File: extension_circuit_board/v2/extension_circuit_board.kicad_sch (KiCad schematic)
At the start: 9 parts, among them J1 GPIO_odd, J2 Jetson_Nano_GPIO, J3 GPIO_even, J4 FeatherWing_DCmotor, J5 PiOLED 2x3, J6 Motor Power, J7 Battery, SW1 SW_SPDT, U1 DFR0753

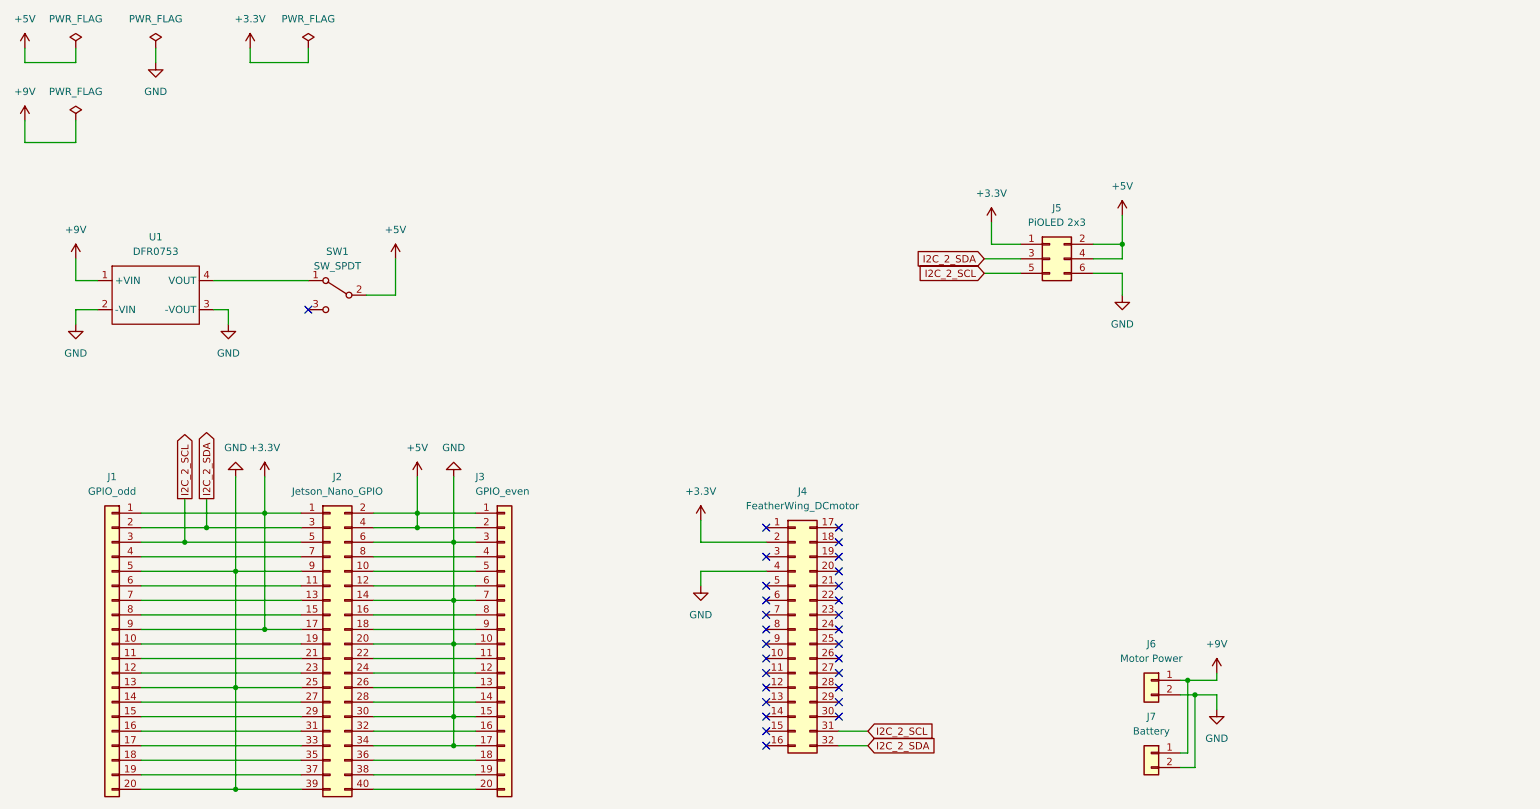
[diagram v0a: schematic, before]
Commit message: Updated
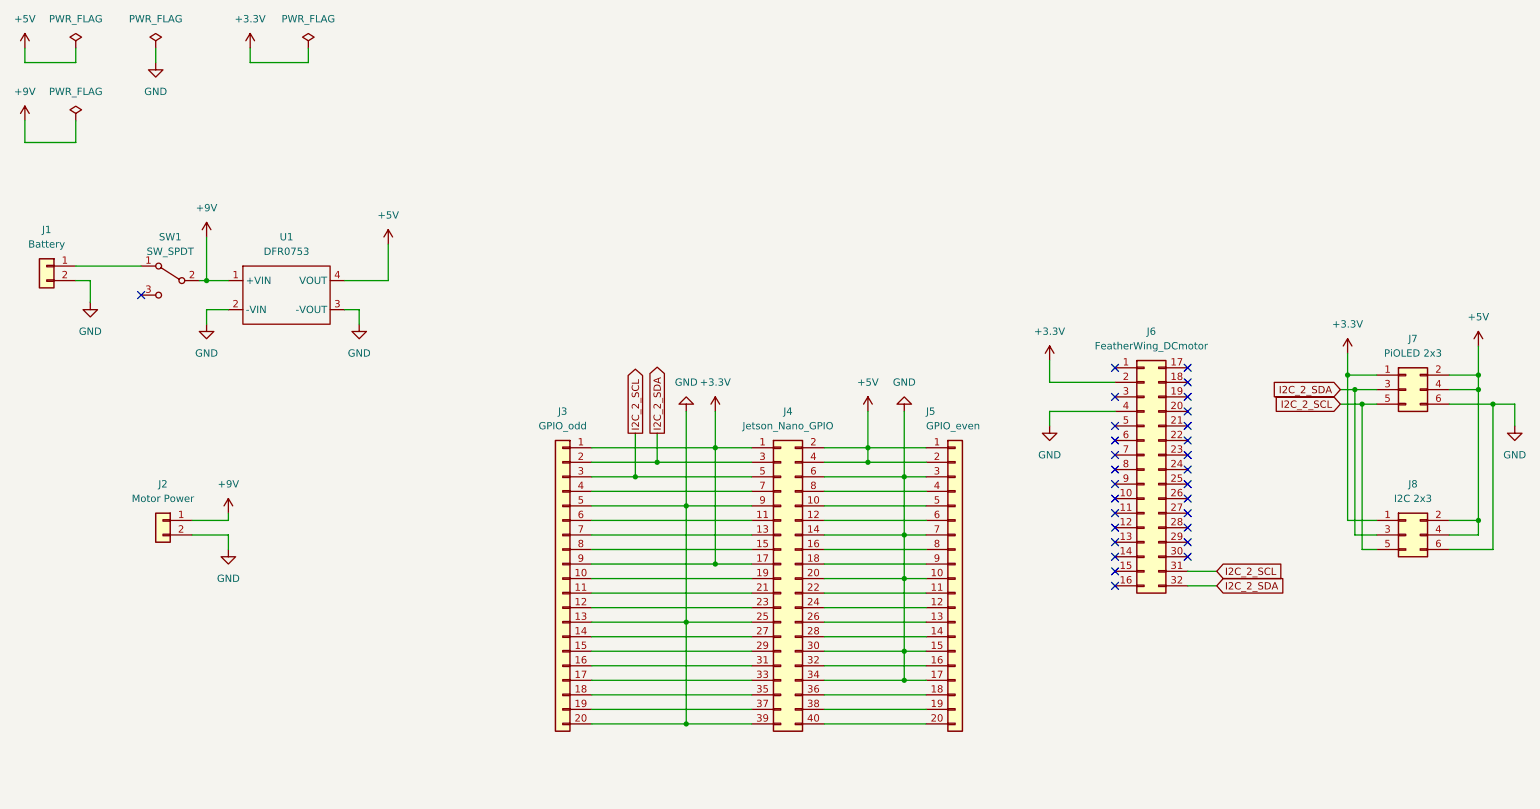
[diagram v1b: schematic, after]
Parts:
- added J8: I2C 2x3, Connector_PinHeader_2.54mm:PinHeader_2x03_P2.54mm_Vertical, symbol Connector_Generic:Conn_02x03_Odd_Even
- renumbered J7 to J1, J6 to J2, J1 to J3, J2 to J4, J3 to J5, J4 to J6, J5 to J7
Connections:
- net +3.3V: now also J8.1 (Pin_1)
- net +5V: now also U1.4 (VOUT), J8.2 (Pin_2), J8.4 (Pin_4); no longer SW1.2 (B)
- net +9V: now also SW1.2 (B); no longer J1.1 (Pin_1)
- net GND: now also J8.6 (Pin_6)
- net I2C_2_SCL: now also J8.5 (Pin_5)
- net I2C_2_SDA: now also J8.3 (Pin_3)
- net at SW1.1 (A): now also J1.1 (Pin_1); no longer U1.4 (VOUT)
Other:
- moved on the sheet: J1, J2, J3, J4, J5, J6, J7, SW1, U1
